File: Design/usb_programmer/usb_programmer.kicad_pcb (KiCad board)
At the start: 4 copper layers, 32.8 x 38.6 mm, 28 parts, among them J1 Conn_01x20_Male, J2 Conn_01x02_Pin, J3 Conn_01x02_Pin, J5 Conn_01x02_Male, J6 Conn_01x02_Male, P1 USB_C_Plug, Q2 BSS138, Q3 BSS138, U1 USB-C-31-M-12

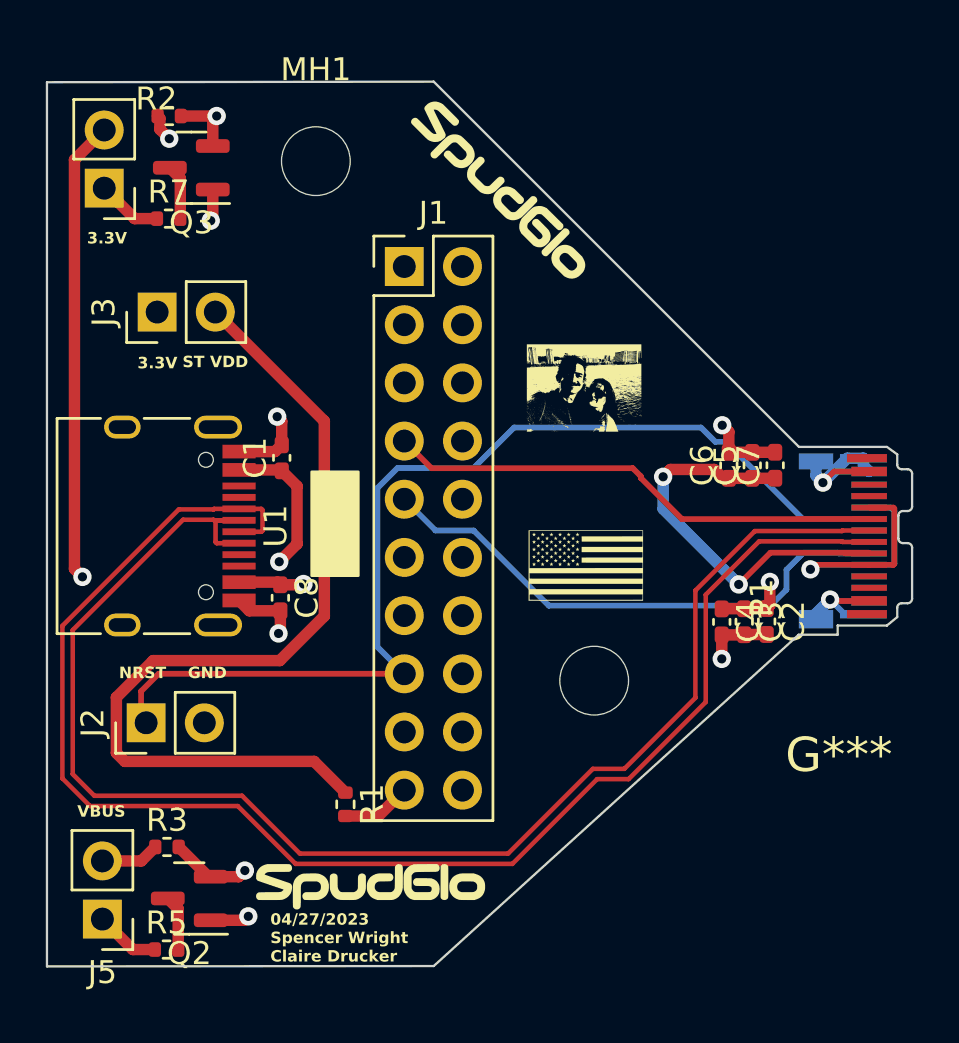
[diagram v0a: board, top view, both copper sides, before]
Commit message: spudglo v6 added
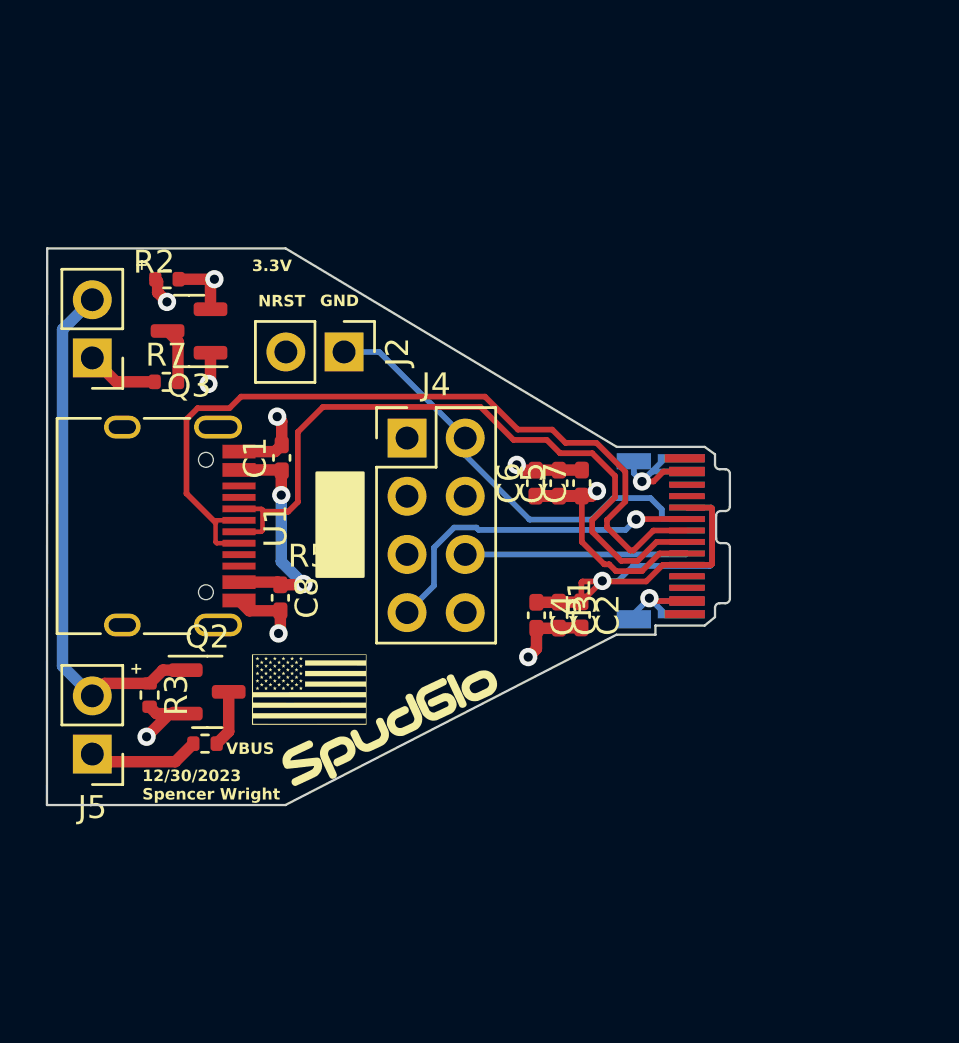
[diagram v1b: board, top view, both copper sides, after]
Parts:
- removed the G*** at (43.9, 62.4)
- removed the G*** at (47.6, 70.9)
- removed J1: Conn_01x20_Male, Connector_PinHeader_2.54mm:PinHeader_2x10_P2.54mm_Vertical
- removed J3: Conn_01x02_Pin, Connector_PinHeader_2.54mm:PinHeader_1x02_P2.54mm_Vertical
- removed MH1, MH2: MountingHole_Pad, MountingHole:MountingHole_3mm
- removed R1: 0, Resistor_SMD:R_0402_1005Metric
- added J4: Conn_01x08_Male, Connector_PinHeader_2.54mm:PinHeader_2x04_P2.54mm_Vertical, F.Cu at (39.9, 73.1)
- moved J2 18.4 mm to (37.1, 69.3), turned to -90 degrees
- moved G*** 13.2 mm to (35.6, 84.1)
- moved R5 9.15 mm to (31.1, 86.5)
- moved Q2 9.05 mm to (31.1, 84.2), turned to 0 degrees
- moved C5 8.47 mm to (46.5, 75.1)
- moved C6 8.47 mm to (45.5, 75.1)
- moved C7 8.47 mm to (47.5, 75.1)
- moved C2 8.10 mm to (47.5, 80.8)
- moved C3 8.10 mm to (46.5, 80.8)
- moved C4 8.10 mm to (45.5, 80.8)
- moved P1 7.95 mm to (50.9, 77.4)
- moved J6 7.43 mm to (26.1, 69.6)
- moved J5 7.22 mm to (26.1, 86.9)
- moved Q3 7.13 mm to (30.4, 68.4)
- moved R2 7.13 mm to (29.4, 66.2)
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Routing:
- net MCU_VDD: track 38.9 -> 0.00 mm
- net USBD-: track 64.8 -> 31.2 mm
- net USBD+: track 63.3 -> 36.0 mm
- net NRST: track 46.1 -> 19.4 mm
- net SWCLK: track 23.7 -> 9.70 mm
- net SWDIO: track 21.7 -> 15.0 mm, vias 0 -> 1
- net +3.3V: track 21.2 -> 15.3 mm, vias 4 -> 3
- net VBUS: track 51.5 -> 55.4 mm, vias 6 -> 3
- net Net-(J1-Pin_19): track 3.04 -> 0.00 mm
- net Net-(J5-Pin_1): track 2.84 -> 4.88 mm
- net GND1: track 33.8 -> 33.1 mm
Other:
- board size 32.8 x 38.6 mm -> 24.9 x 24.3 mm
- board text added: "+"
- board text added: "12/30/2023 Spencer Wright"
- board text removed: "04/27/2023 Spencer Wright Claire Drucker"
- board text removed: "ST VDD"
